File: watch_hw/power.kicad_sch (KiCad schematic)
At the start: 14 parts, among them U2 nPM1100-QDAA, U3 MAX17048G+

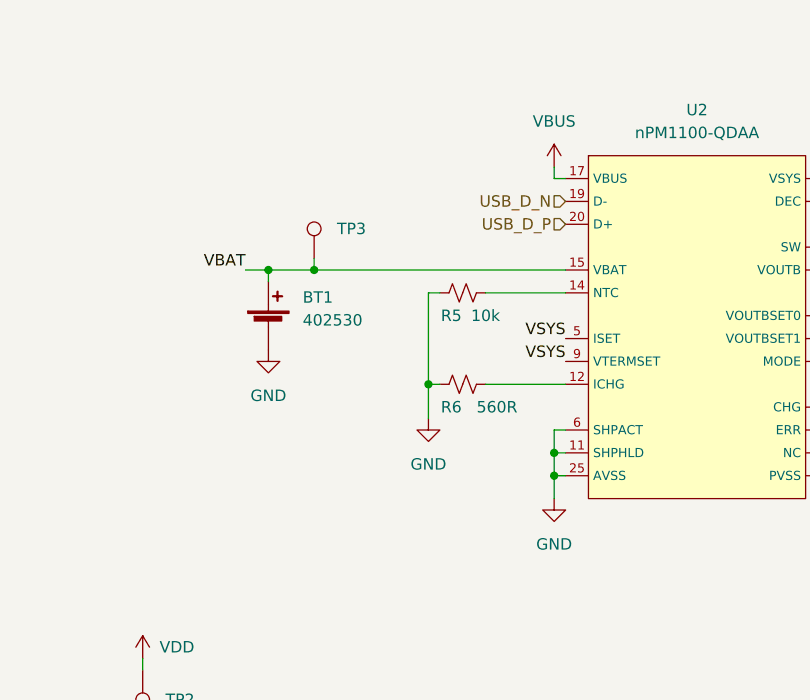
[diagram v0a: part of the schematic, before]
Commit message: finish routing, need to fix DRC
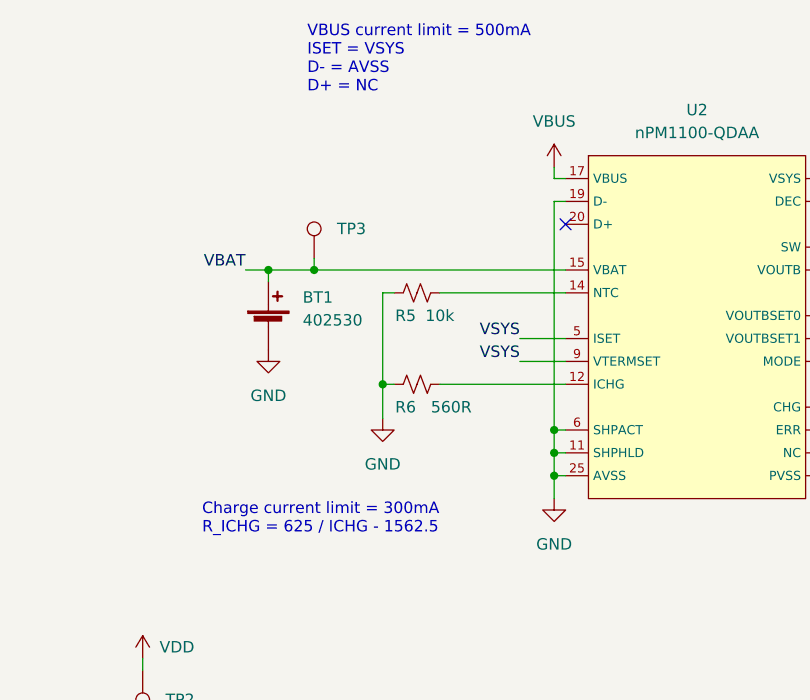
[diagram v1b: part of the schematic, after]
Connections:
- net USB_D_N is gone; now on net GND: U2.19 (D-)
- net USB_D_P: no longer names the net of U2.20 (D+)
- no-connect marks 0 -> 1
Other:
- note added: "Charge current limit = 300mA R_ICHG = 625 / ICHG - 1562.5"
- note added: "VBUS current limit = 500mA ISET = VSYS D- = AVSS D+ = NC"
- moved on the sheet: R5, R6
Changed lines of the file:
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@@
 	(generator_version "9.0")
 	(paper "A4")
+	(text "Charge current limit = 300mA\nR_ICHG = 625 / ICHG - 1562.5"
+		(exclude_from_sim no)
+		(at 146.304 111.506 0)
+		(effects
+			(font
+				(size 1.27 1.27)
+			)
+			(justify left)
+		)
+	)
+	(text "VBUS current limit = 500mA\nISET = VSYS\nD- = AVSS\nD+ = NC"
+		(exclude_from_sim no)
+		(at 157.988 60.452 0)
+		(effects
+			(font
+				(size 1.27 1.27)
+			)
+			(justify left)
+		)
+	)
+	(junction
+		(at 185.42 101.6)
+		(diameter 0)
+		(color 0 0 0 0)
+	)
 	(junction
 		(at 242.57 73.66)
@@
 	)
 	(junction
-		(at 171.45 96.52)
+		(at 166.37 96.52)
 		(diameter 0)
 		(color 0 0 0 0)
 	)
+	(no_connect
+		(at 186.69 78.74)
+	)
 	(wire
 		(pts
@@
 	(wire
 		(pts
+			(xy 185.42 76.2) (xy 185.42 101.6)
+		)
+		(stroke
+			(width 0)
+			(type default)
+		)
+	)
+	(wire
+		(pts
 			(xy 102.87 82.55) (xy 104.14 82.55)
 		)
@@
 	(wire
 		(pts
+			(xy 181.61 93.98) (xy 186.69 93.98)
+		)
+		(stroke
+			(width 0)
+			(type default)
+		)
+	)
+	(wire
+		(pts
 			(xy 60.96 85.09) (xy 60.96 87.63)
 		)
@@
 	(wire
 		(pts
-			(xy 171.45 96.52) (xy 171.45 100.33)
+			(xy 166.37 96.52) (xy 166.37 100.33)
 		)
 		(stroke
@@
 	(wire
 		(pts
+			(xy 181.61 91.44) (xy 186.69 91.44)
+		)
+		(stroke
+			(width 0)
+			(type default)
+		)
+	)
+	(wire
+		(pts
 			(xy 59.69 82.55) (xy 62.23 82.55)
 		)
@@
 	(wire
 		(pts
-			(xy 171.45 96.52) (xy 172.72 96.52)
+			(xy 166.37 96.52) (xy 167.64 96.52)
 		)
 		(stroke
@@
 	(wire
 		(pts
+			(xy 186.69 76.2) (xy 185.42 76.2)
+		)
+		(stroke
+			(width 0)
+			(type default)
+		)
+	)
+	(wire
+		(pts
 			(xy 104.14 90.17) (xy 102.87 90.17)
 		)
@@
 	(wire
 		(pts
-			(xy 177.8 96.52) (xy 186.69 96.52)
-		)
-		(stroke
-			(width 0)
-			(type default)
-		)
-	)
-	(wire
-		(pts
-			(xy 171.45 86.36) (xy 171.45 96.52)
+			(xy 172.72 96.52) (xy 186.69 96.52)
+		)
+		(stroke
+			(width 0)
+			(type default)
+		)
+	)
+	(wire
+		(pts
+			(xy 166.37 86.36) (xy 166.37 96.52)
 		)
 		(stroke
@@
 	(wire
 		(pts
-			(xy 172.72 86.36) (xy 171.45 86.36)
+			(xy 167.64 86.36) (xy 166.37 86.36)
 		)
 		(stroke
@@
 	(wire
 		(pts
-			(xy 177.8 86.36) (xy 186.69 86.36)
+			(xy 172.72 86.36) (xy 186.69 86.36)
 		)
 		(stroke
@@
 	)
 	(label "VSYS"
-		(at 186.69 91.44 180)
+		(at 181.61 91.44 180)
 		(effects
 			(font
@@
 	)
 	(label "VSYS"
-		(at 186.69 93.98 180)
+		(at 181.61 93.98 180)
 		(effects
 			(font
@@
 		)
 	)
-	(hierarchical_label "USB_D_P"
-		(shape input)
-		(at 186.69 78.74 180)
-		(effects
-			(font
-				(size 1.27 1.27)
-			)
-			(justify right)
-		)
-	)
-	(hierarchical_label "USB_D_N"
-		(shape input)
-		(at 186.69 76.2 180)
-		(effects
-			(font
-				(size 1.27 1.27)
-			)
-			(justify right)
-		)
-	)
 	(symbol
 		(lib_id "power:VBUS")
@@
 		(lib_name "GND_1")
 		(lib_id "power:GND")
-		(at 171.45 100.33 0)
+		(at 166.37 100.33 0)
 		(unit 1)
 		(exclude_from_sim no)
@@
 		(fields_autoplaced yes)
 		(property "Reference" "#PWR042"
-			(at 171.45 106.68 0)
+			(at 166.37 106.68 0)
 			(effects
 				(font
@@
 		)
 		(property "Value" "GND"
-			(at 171.45 105.41 0)
+			(at 166.37 105.41 0)
 			(effects
 				(font
@@
 		)
 		(property "Footprint" ""
-			(at 171.45 100.33 0)
+			(at 166.37 100.33 0)
 			(effects
 				(font
@@
 		)
 		(property "Datasheet" ""
-			(at 171.45 100.33 0)
+			(at 166.37 100.33 0)
 			(effects
 				(font
@@
 		)
 		(property "Description" ""
-			(at 171.45 100.33 0)
+			(at 166.37 100.33 0)
 			(effects
 				(font
@@
 			)
 		)
-		(property "Datasheet" "https://infocenter.nordicsemi.com/pdf/nPM1100_PS_v1.3.pdf"
+		(property "Datasheet" "https://docs-be.nordicsemi.com/bundle/ps_npm1100/page/nPM1100_PS_v1.5.pdf"
 			(at 187.96 73.66 0)
 			(effects
@@
 	(symbol
 		(lib_id "Device:R_Small_US")
-		(at 175.26 86.36 90)
+		(at 170.18 86.36 90)
 		(unit 1)
 		(exclude_from_sim no)
@@
 		(dnp no)
 		(property "Reference" "R5"
-			(at 173.99 88.9 90)
+			(at 168.91 88.9 90)
 			(effects
 				(font
@@
 		)
 		(property "Value" "10k"
-			(at 177.8 88.9 90)
+			(at 172.72 88.9 90)
 			(effects
 				(font
@@
 		)
 		(property "Footprint" "Resistor_SMD:R_0402_1005Metric_Pad0.72x0.64mm_HandSolder"
-			(at 175.26 86.36 0)
+			(at 170.18 86.36 0)
 			(effects
 				(font
@@
 		)
 		(property "Datasheet" "~"
-			(at 175.26 86.36 0)
+			(at 170.18 86.36 0)
 			(effects
 				(font
@@
 		)
 		(property "Description" ""
-			(at 175.26 86.36 0)
+			(at 170.18 86.36 0)
 			(effects
 				(font
@@
 	(symbol
 		(lib_id "Device:R_Small_US")
-		(at 175.26 96.52 90)
+		(at 170.18 96.52 90)
 		(unit 1)
 		(exclude_from_sim no)
@@
 		(dnp no)
 		(property "Reference" "R6"
+			(at 168.91 99.06 90)
+			(effects
+				(font
+					(size 1.27 1.27)
+				)
+			)
+		)
+		(property "Value" "560R"
 			(at 173.99 99.06 90)
 			(effects
@@
 			)
 		)
-		(property "Value" "560R"
-			(at 179.07 99.06 90)
-			(effects
-				(font
-					(size 1.27 1.27)
-				)
-			)
-		)
 		(property "Footprint" "Resistor_SMD:R_0402_1005Metric_Pad0.72x0.64mm_HandSolder"
-			(at 175.26 96.52 0)
+			(at 170.18 96.52 0)
 			(effects
 				(font
@@
 		)
 		(property "Datasheet" "~"
-			(at 175.26 96.52 0)
+			(at 170.18 96.52 0)
 			(effects
 				(font
@@
 		)
 		(property "Description" ""
-			(at 175.26 96.52 0)
-			(effects
-				(font
+			(at 170.18 96.52 0)
+			(effects
+				(font
